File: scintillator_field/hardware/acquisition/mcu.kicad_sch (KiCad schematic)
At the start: 1 part, among them U2 STM32F411CEUx

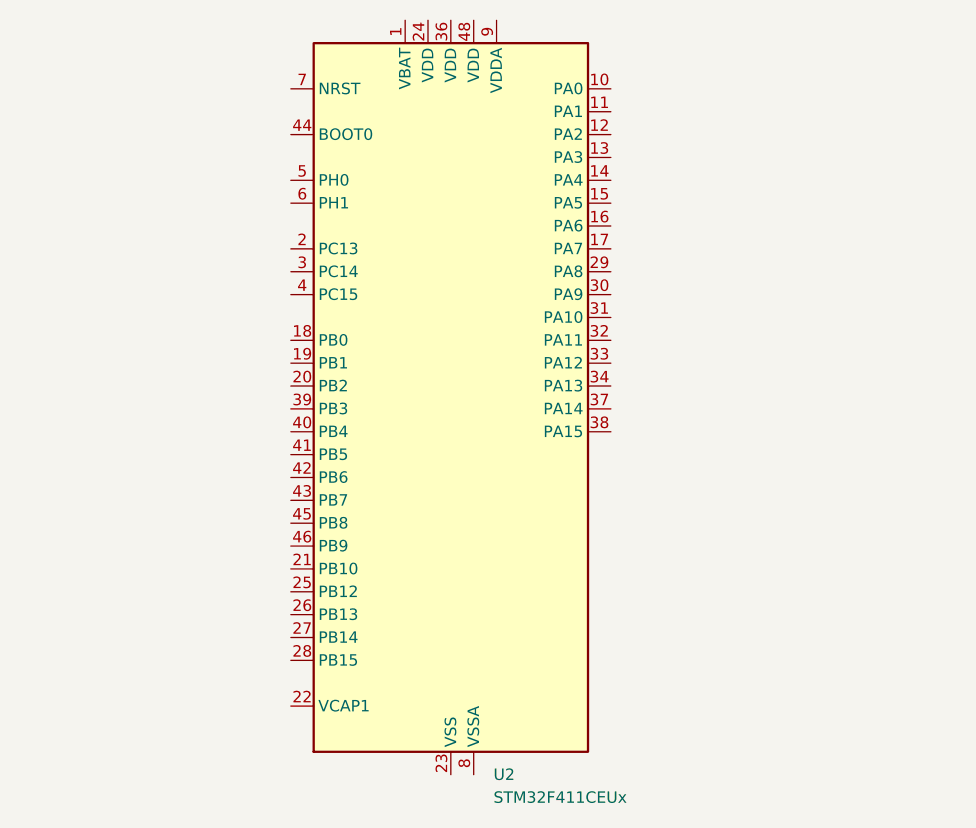
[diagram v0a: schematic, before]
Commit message: usb-c
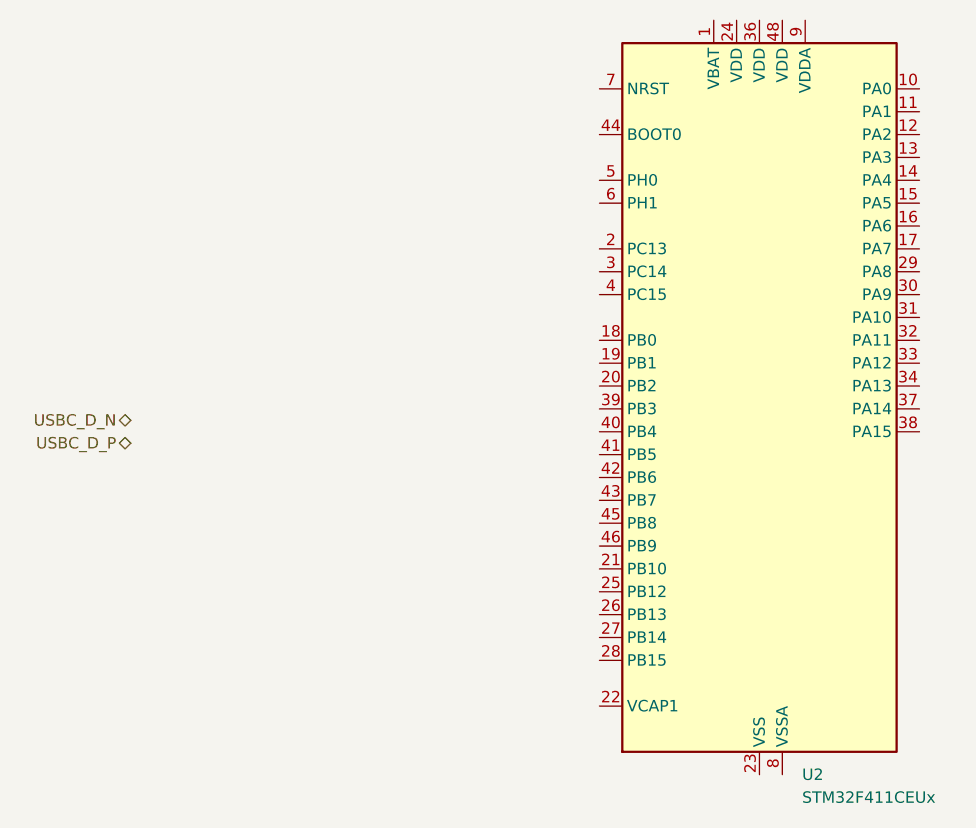
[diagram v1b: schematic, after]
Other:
- moved on the sheet: U2
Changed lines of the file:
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@@
 	(generator_version "8.0")
 	(paper "A4")
+	(hierarchical_label "USBC_D_N"
+		(shape bidirectional)
+		(at 44.45 87.63 180)
+		(fields_autoplaced yes)
+		(effects
+			(font
+				(size 1.27 1.27)
+			)
+			(justify right)
+		)
+	)
+	(hierarchical_label "USBC_D_P"
+		(shape bidirectional)
+		(at 44.45 90.17 180)
+		(fields_autoplaced yes)
+		(effects
+			(font
+				(size 1.27 1.27)
+			)
+			(justify right)
+		)
+	)
 	(symbol
 		(lib_id "MCU_ST_STM32F4:STM32F411CEUx")
-		(at 80.01 86.36 0)
+		(at 114.3 86.36 0)
 		(unit 1)
 		(exclude_from_sim no)
@@
 		(fields_autoplaced yes)
 		(property "Reference" "U2"
-			(at 84.7441 127 0)
+			(at 119.0341 127 0)
 			(effects
 				(font
@@
 		)
 		(property "Value" "STM32F411CEUx"
-			(at 84.7441 129.54 0)
+			(at 119.0341 129.54 0)
 			(effects
 				(font
@@
 		)
 		(property "Footprint" "Package_DFN_QFN:QFN-48-1EP_7x7mm_P0.5mm_EP5.6x5.6mm"
-			(at 64.77 124.46 0)
+			(at 99.06 124.46 0)
 			(effects
 				(font
@@
 		)
 		(property "Datasheet" "https://www.st.com/resource/en/datasheet/stm32f411ce.pdf"
-			(at 80.01 86.36 0)
+			(at 114.3 86.36 0)
 			(effects
 				(font
@@
 		)
 		(property "Description" "STMicroelectronics Arm Cortex-M4 MCU, 512KB flash, 128KB RAM, 100 MHz, 1.7-3.6V, 36 GPIO, UFQFPN48"
-			(at 80.01 86.36 0)
+			(at 114.3 86.36 0)
 			(effects
 				(font
